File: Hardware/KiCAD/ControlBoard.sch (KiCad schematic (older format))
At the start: 1 part

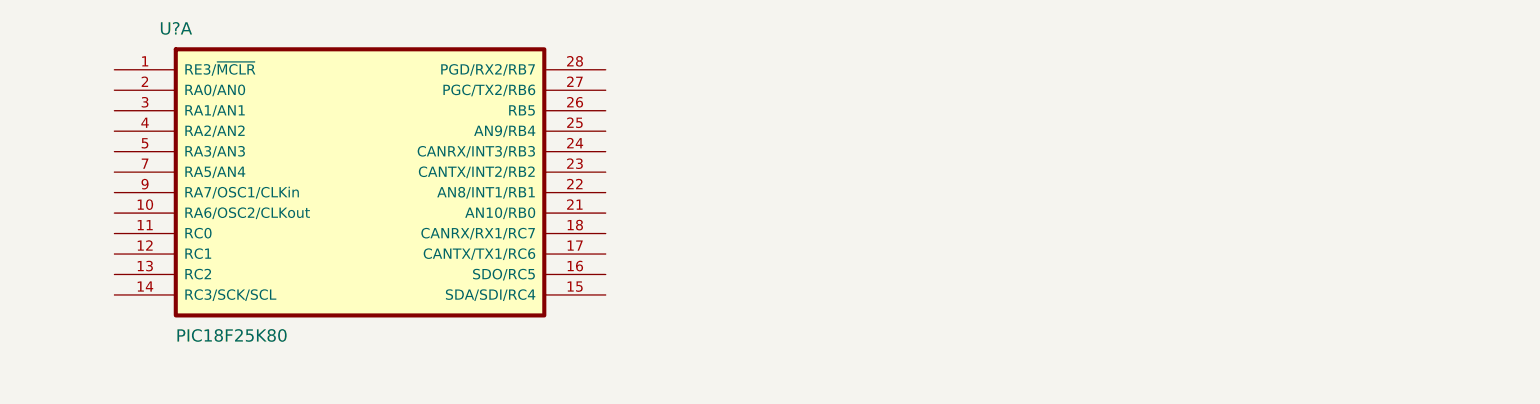
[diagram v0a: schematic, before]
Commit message: First commit of KiCAD project
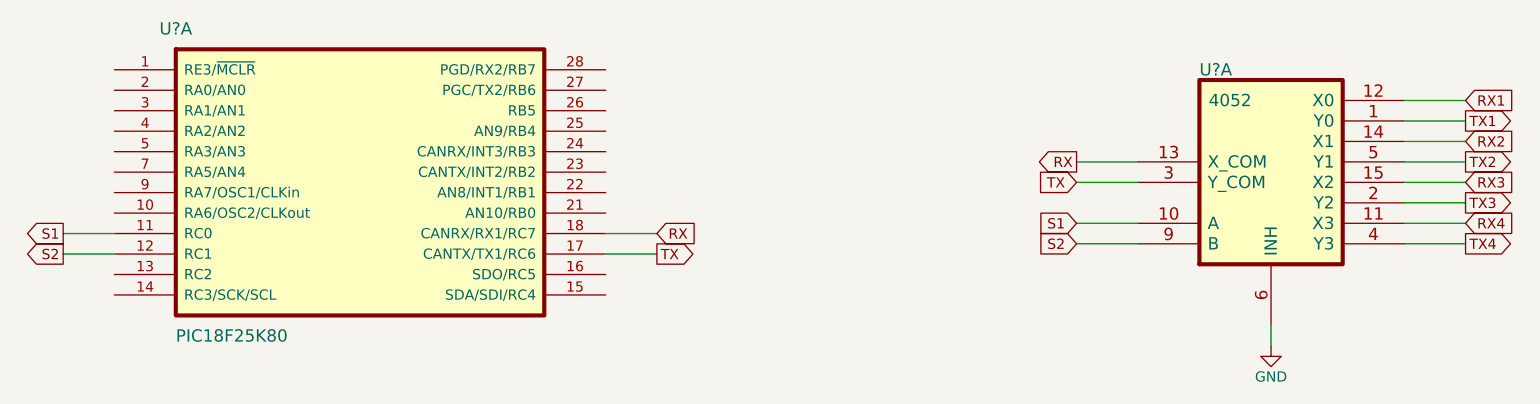
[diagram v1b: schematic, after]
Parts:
- added U?: 4000series-4052, DIP16, symbol 4000series-4052
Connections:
- net S1: now reaches U?.11 (RC0)
- net S1: now also U?.10 (A)
- net S2: now reaches U?.12 (RC1)
- net S2: now also U?.9 (B)
- net TX: now reaches U?.17 (CANTX/TX1/RC6)
- net TX: now also U?.3 (Y_COM)
- net RX: now reaches U?.18 (CANRX/RX1/RC7)
- net RX: now also U?.13 (X_COM)
- new net GND: U?.6 (INH)
- new net RX1: U?.12 (X0)
- new net RX2: U?.14 (X1)
- new net RX3: U?.15 (X2)
- new net RX4: U?.11 (X3)
- new net TX1: U?.1 (Y0)
- new net TX2: U?.5 (Y1)
- new net TX3: U?.2 (Y2)
- new net TX4: U?.4 (Y3)
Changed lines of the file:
@@
 	1    0    0    -1
 $EndComp
+$Comp
+L 4000series-4052 U?
+U 1 1 57AA0379
+P 10200 3300
+F 0 "U?" H 9850 3800 60  0000 L CNN
+F 1 "4000series-4052" H 9850 3900 60  0001 L CNN
+F 2 "DIP16" H 10400 3250 60  0001 C CNN
+F 3 "" H 10400 3250 60  0000 C CNN
+F 4 "4052" H 10000 3650 60  0000 C CNN "Device"
+	1    10200 3300
+	1    0    0    -1
+$EndComp
+Text GLabel 11150 2950 2    50   Input ~ 0
+RX1
+Text GLabel 11150 3150 2    50   Input ~ 0
+RX2
+Text GLabel 11150 3350 2    50   Input ~ 0
+RX3
+Text GLabel 11150 3550 2    50   Input ~ 0
+RX4
+Text GLabel 11150 3050 2    50   Output ~ 0
+TX1
+Text GLabel 11150 3250 2    50   Output ~ 0
+TX2
+Text GLabel 11150 3450 2    50   Output ~ 0
+TX3
+Text GLabel 11150 3650 2    50   Output ~ 0
+TX4
+Text GLabel 9250 3250 0    50   Output ~ 0
+RX
+Text GLabel 9250 3350 0    50   Input ~ 0
+TX
+Text GLabel 7200 3700 2    50   Output ~ 0
+TX
+Text GLabel 7200 3600 2    50   Input ~ 0
+RX
+Text GLabel 4300 3600 0    50   Output ~ 0
+S1
+Text GLabel 4300 3700 0    50   Output ~ 0
+S2
+Text GLabel 9250 3550 0    50   Input ~ 0
+S1
+Text GLabel 9250 3650 0    50   Input ~ 0
+S2
+Wire Wire Line
+	11150 2950 10850 2950
+Wire Wire Line
+	11150 3050 10850 3050
+Wire Wire Line
+	10850 3150 11150 3150
+Wire Wire Line
+	10850 3250 11150 3250
+Wire Wire Line
+	10850 3350 11150 3350
+Wire Wire Line
+	11150 3450 10850 3450
+Wire Wire Line
+	10850 3550 11150 3550
+Wire Wire Line
+	11150 3650 10850 3650
+Wire Wire Line
+	9250 3250 9550 3250
+Wire Wire Line
+	9250 3350 9550 3350
+Wire Wire Line
+	7200 3700 6950 3700
+Wire Wire Line
+	7200 3600 6950 3600
+Wire Wire Line
+	4300 3600 4550 3600
+Wire Wire Line
+	4550 3700 4300 3700
+Wire Wire Line
+	9250 3550 9550 3550
+Wire Wire Line
+	9550 3650 9250 3650
+$Comp
+L GND #PWR?
+U 1 1 57AA0898
+P 10200 4150
+F 0 "#PWR?" H 10200 3900 50  0001 C CNN
+F 1 "GND" H 10200 4000 50  0000 C CNN
+F 2 "" H 10200 4150 50  0000 C CNN
+F 3 "" H 10200 4150 50  0000 C CNN
+	1    10200 4150
+	1    0    0    -1
+$EndComp
+Wire Wire Line
+	10200 4150 10200 4050
 $EndSCHEMATC
